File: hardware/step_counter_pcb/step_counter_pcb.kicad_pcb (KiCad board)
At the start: 2 copper layers, 65 x 40 mm, 29 parts, among them J1 LiPo_Battery, J2 USB_C_Receptacle_USB2.0_16P, SW1 SW_SPST, SW2 SW_Push, U1 TPS63031DSK, U2 ESP32-C3-MINI-1, U3 LIS2DUX12, U4 EEPROM, U5 ER_OLEDM0.91_1x-I2C, U6 TPD2EUSB30

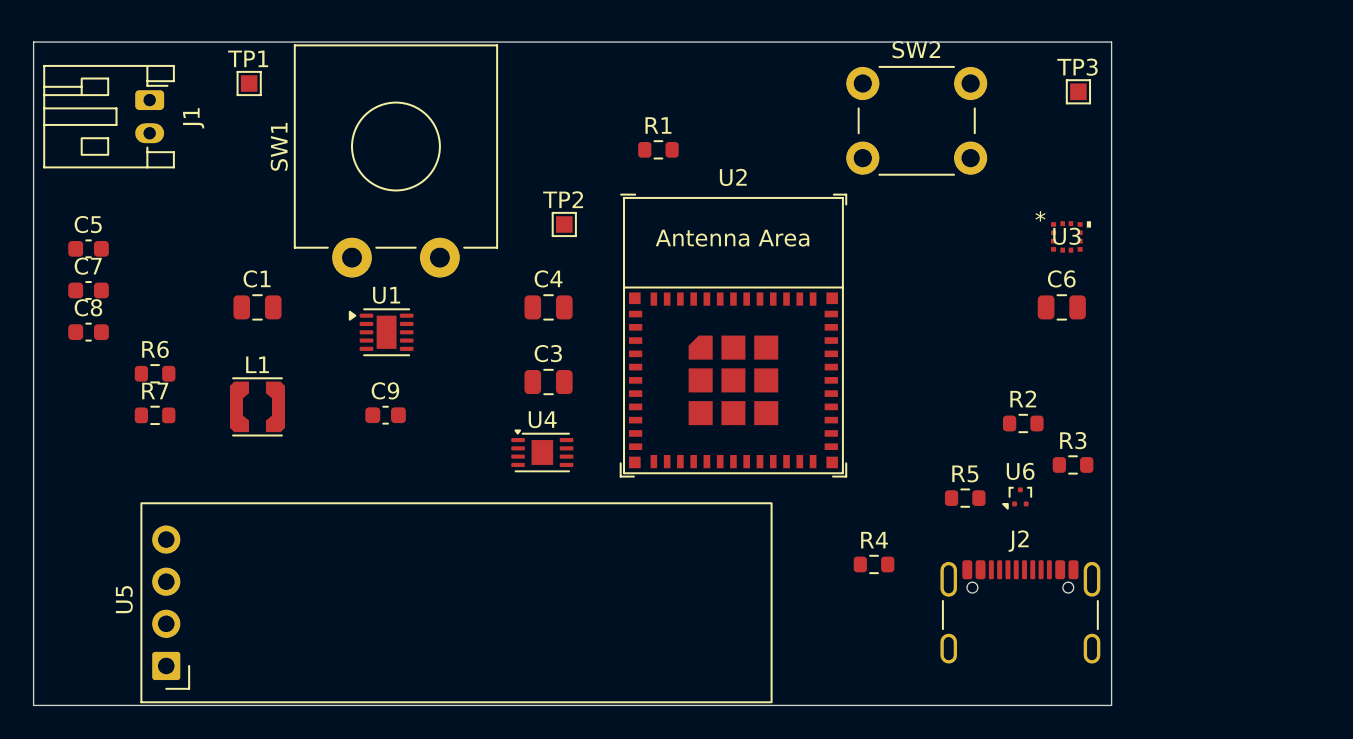
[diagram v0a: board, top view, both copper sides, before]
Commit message: Updates layout
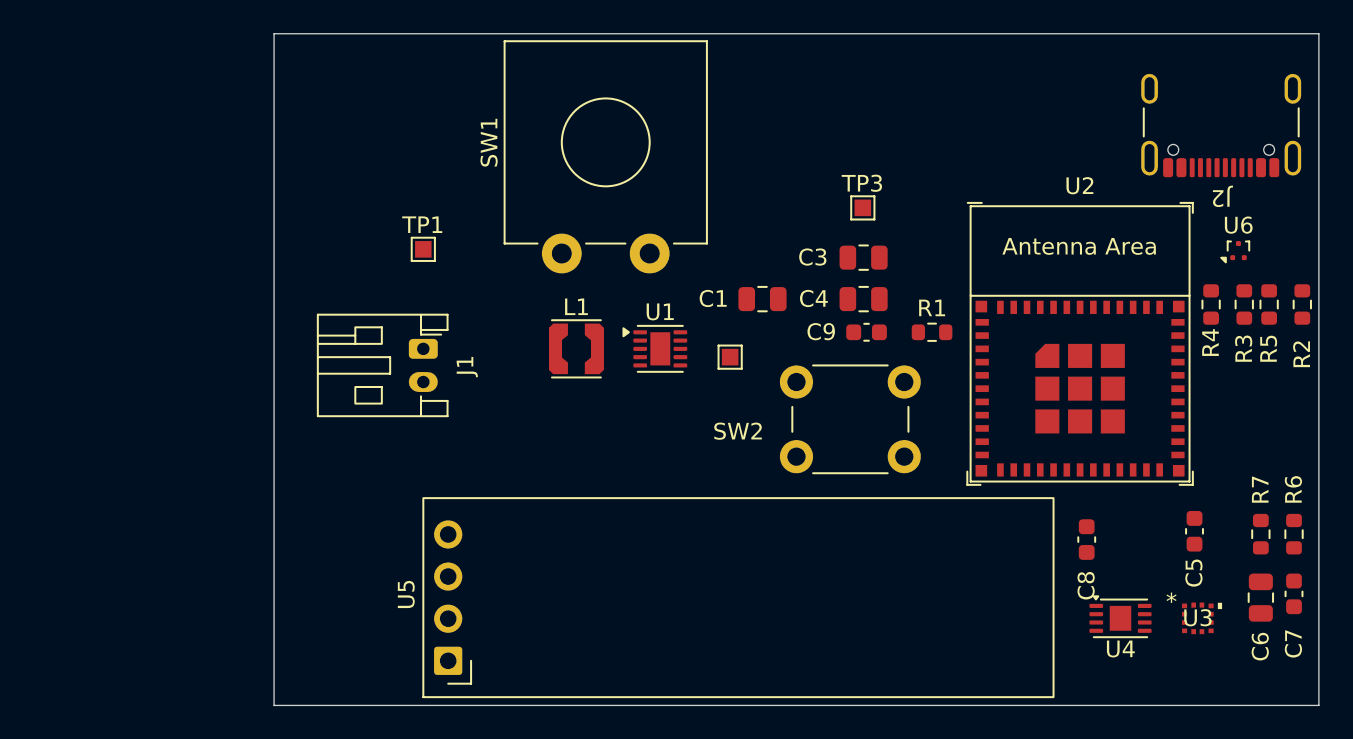
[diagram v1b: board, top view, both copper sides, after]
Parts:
- moved C7 75.0 mm to (126.0, 83.3), turned to 90 degrees
- moved R6 69.4 mm to (126.0, 79.7), turned to 90 degrees
- moved C5 68.8 mm to (120.0, 79.5), turned to 90 degrees
- moved R7 67.1 mm to (124.0, 79.7), turned to 90 degrees
- moved C8 61.5 mm to (113.5, 80.0), turned to -90 degrees
- moved U4 36.3 mm to (115.5, 84.8)
- moved J2 33.8 mm to (121.6, 53.9), turned to 180 degrees
- moved C1 30.5 mm to (94.0, 65.5)
- moved C9 29.4 mm to (100.2, 67.5)
- moved R4 25.7 mm to (121.0, 65.8), turned to 90 degrees
- moved U3 24.3 mm to (120.2, 84.7)
- moved J1 22.3 mm to (73.5, 68.5)
- moved R5 21.7 mm to (124.5, 65.8), turned to 90 degrees
- moved C6 21.2 mm to (124.0, 83.5), turned to 90 degrees
- moved U2 20.9 mm to (113.1, 68.2)
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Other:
- board size 65 x 40 mm -> 63 x 40.5 mm
